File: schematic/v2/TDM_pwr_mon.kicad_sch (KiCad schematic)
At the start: 42 parts, among them J10 INA219_CONFIG, J11 INA219_CONFIG, J15 INA219_CONFIG, J5 INA219_CONFIG, J6 INA219_CONFIG, J7 INA219_CONFIG, U10 INA219AxD, U11 INA219AxD, U12 INA219AxD, U13 INA219AxD, U20 INA219AxD, U7 INA219AxD

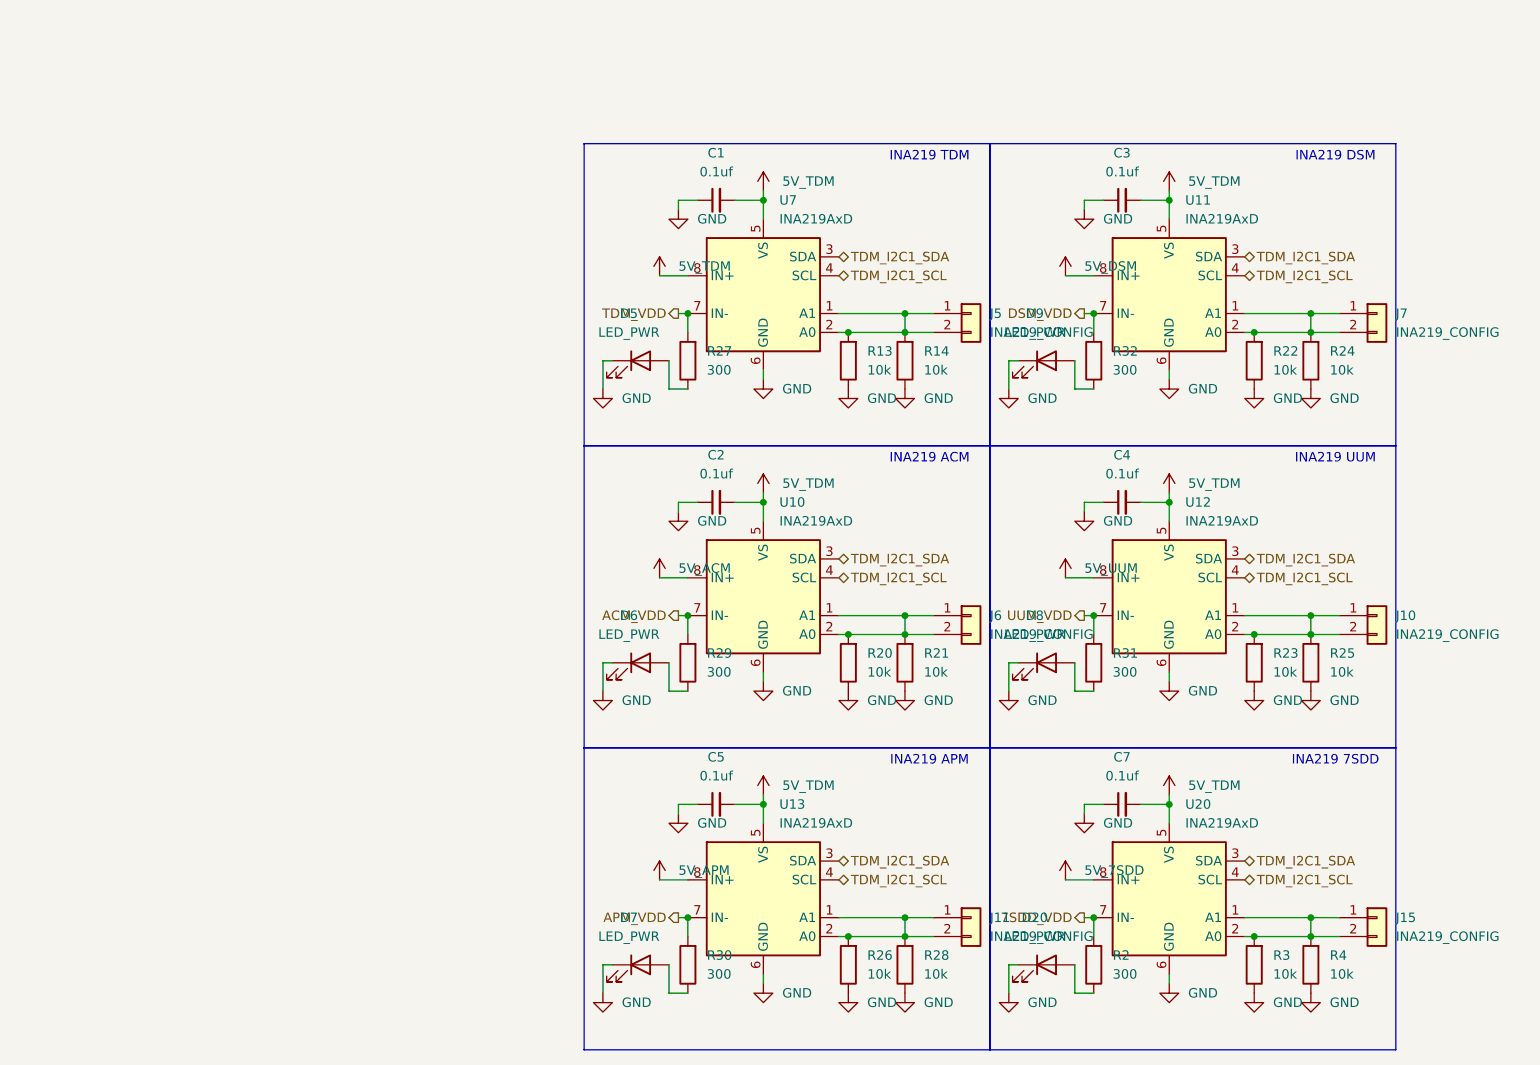
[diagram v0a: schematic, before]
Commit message: no errors in the ERC!
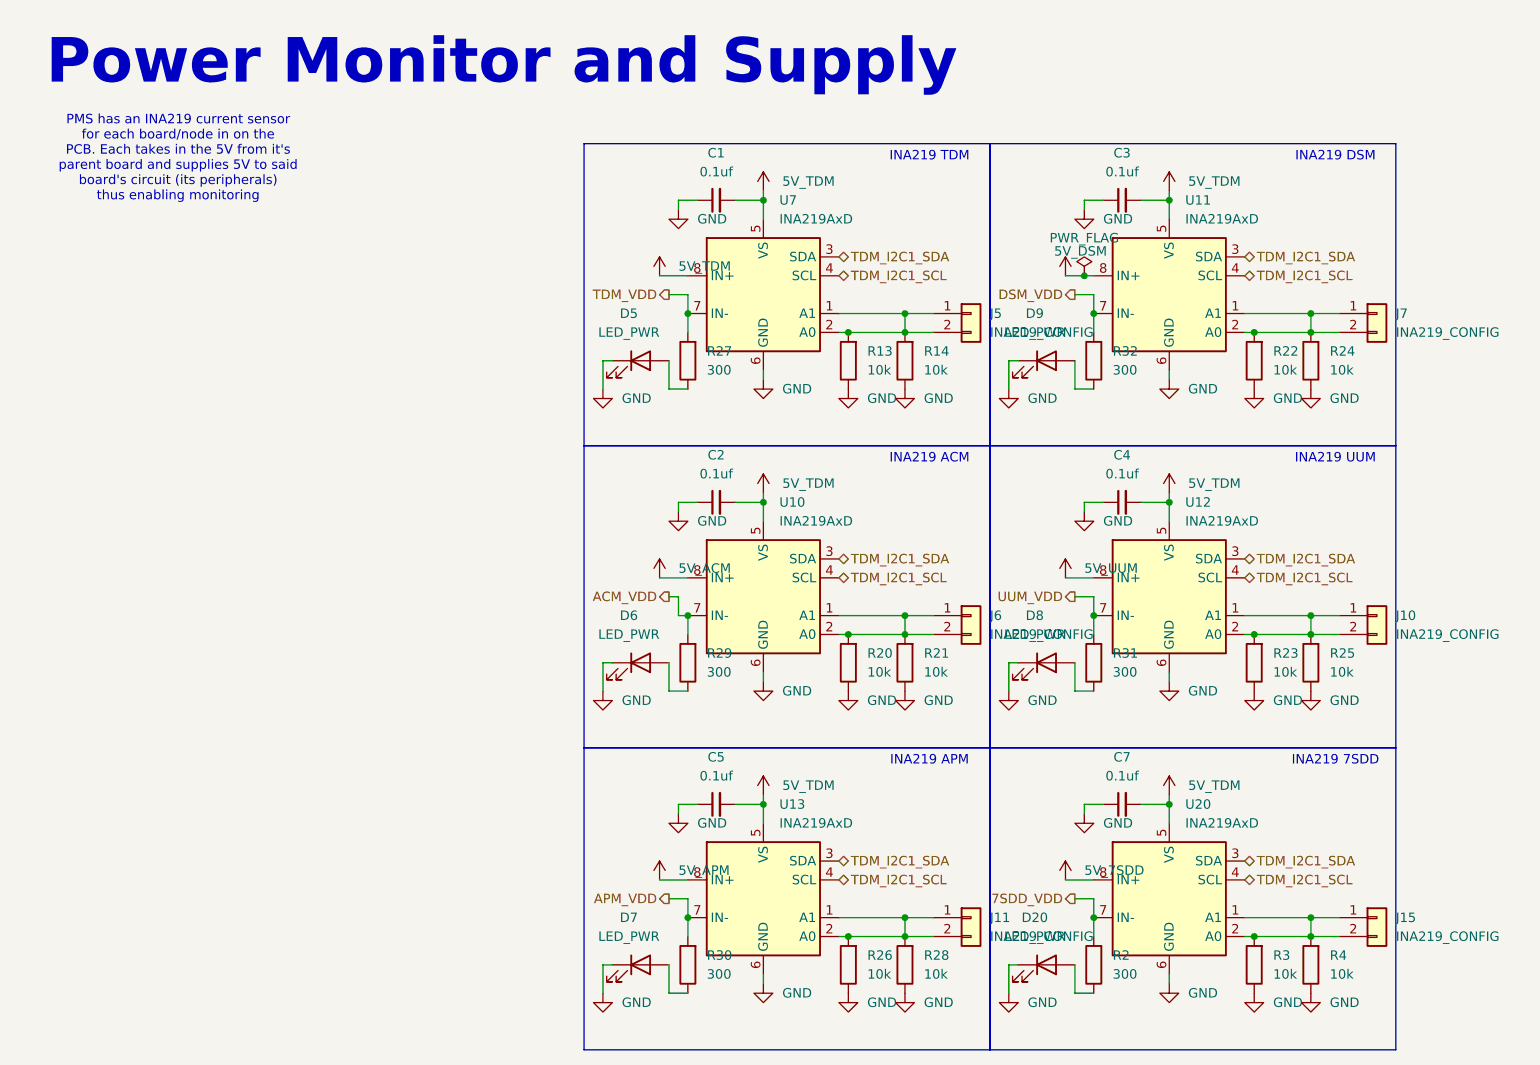
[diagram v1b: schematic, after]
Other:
- note added: "PMS has an INA219 current sensor for each board/node in on the PCB. Each takes in the 5V from it's parent board and supplies 5V to said board's circuit (its peripherals) thus enabling monitoring"
- note added: "Power Monitor and Supply"
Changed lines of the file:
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@@
 		)
 	)
+	(text "PMS has an INA219 current sensor\nfor each board/node in on the \nPCB. Each takes in the 5V from it's\nparent board and supplies 5V to said\nboard's circuit (its peripherals)\nthus enabling monitoring"
+		(exclude_from_sim no)
+		(at 34.29 32.512 0)
+		(effects
+			(font
+				(size 1.27 1.27)
+			)
+		)
+	)
 	(text "INA219 ACM"
 		(exclude_from_sim no)
@@
 		)
 	)
+	(text "Power Monitor and Supply"
+		(exclude_from_sim no)
+		(at 16.51 23.114 0)
+		(effects
+			(font
+				(size 5.9944 5.9944)
+				(thickness 1.1989)
+				(bold yes)
+			)
+			(justify left bottom)
+		)
+	)
 	(text "INA219 UUM"
 		(exclude_from_sim no)
@@
 	)
 	(junction
+		(at 156.21 48.26)
+		(diameter 0)
+		(color 0 0 0 0)
+	)
+	(junction
 		(at 186.69 93.98)
 		(diameter 0)
@@
 	(wire
 		(pts
-			(xy 153.67 48.26) (xy 157.48 48.26)
+			(xy 167.64 38.1) (xy 167.64 40.64)
+		)
+		(stroke
+			(width 0)
+			(type default)
+		)
+	)
+	(wire
+		(pts
+			(xy 153.67 48.26) (xy 156.21 48.26)
 		)
 		(stroke
@@
 	(wire
 		(pts
-			(xy 163.83 78.74) (xy 167.64 78.74)
+			(xy 156.21 48.26) (xy 157.48 48.26)
 		)
 		(stroke
@@
 	(wire
 		(pts
-			(xy 101.6 134.62) (xy 102.87 134.62)
+			(xy 157.48 132.08) (xy 157.48 134.62)
+		)
+		(stroke
+			(width 0)
+			(type default)
+		)
+	)
+	(wire
+		(pts
+			(xy 163.83 78.74) (xy 167.64 78.74)
 		)
 		(stroke
@@
 	(wire
 		(pts
+			(xy 102.87 132.08) (xy 102.87 134.62)
+		)
+		(stroke
+			(width 0)
+			(type default)
+		)
+	)
+	(wire
+		(pts
 			(xy 154.94 59.69) (xy 154.94 63.5)
 		)
@@
 	(wire
 		(pts
+			(xy 157.48 91.44) (xy 157.48 93.98)
+		)
+		(stroke
+			(width 0)
+			(type default)
+		)
+	)
+	(wire
+		(pts
 			(xy 100.33 63.5) (xy 102.87 63.5)
 		)
@@
 	(wire
 		(pts
-			(xy 156.21 53.34) (xy 157.48 53.34)
+			(xy 154.94 50.8) (xy 157.48 50.8)
 		)
 		(stroke
@@
 	(wire
 		(pts
-			(xy 167.64 118.11) (xy 167.64 119.38)
+			(xy 99.06 88.9) (xy 102.87 88.9)
 		)
 		(stroke
@@
 	(wire
 		(pts
-			(xy 177.8 137.16) (xy 179.07 137.16)
+			(xy 167.64 118.11) (xy 167.64 119.38)
 		)
 		(stroke
@@
 	(wire
 		(pts
-			(xy 113.03 101.6) (xy 113.03 102.87)
+			(xy 177.8 137.16) (xy 179.07 137.16)
 		)
 		(stroke
@@
 	(wire
 		(pts
-			(xy 123.19 96.52) (xy 124.46 96.52)
+			(xy 113.03 101.6) (xy 113.03 102.87)
 		)
 		(stroke
@@
 	(wire
 		(pts
-			(xy 153.67 88.9) (xy 157.48 88.9)
+			(xy 123.19 96.52) (xy 124.46 96.52)
 		)
 		(stroke
@@
 	(wire
 		(pts
-			(xy 167.64 38.1) (xy 167.64 40.64)
-		)
-		(stroke
-			(width 0)
-			(type default)
-		)
-	)
-	(wire
-		(pts
 			(xy 91.44 100.33) (xy 92.71 100.33)
 		)
@@
 	(wire
 		(pts
-			(xy 156.21 134.62) (xy 157.48 134.62)
+			(xy 154.94 132.08) (xy 157.48 132.08)
 		)
 		(stroke
@@
 	(wire
 		(pts
-			(xy 156.21 93.98) (xy 157.48 93.98)
+			(xy 154.94 91.44) (xy 157.48 91.44)
 		)
 		(stroke
@@
 	(wire
 		(pts
-			(xy 101.6 53.34) (xy 102.87 53.34)
+			(xy 100.33 50.8) (xy 102.87 50.8)
 		)
 		(stroke
@@
 	(wire
 		(pts
-			(xy 101.6 93.98) (xy 102.87 93.98)
+			(xy 100.33 91.44) (xy 101.6 91.44)
 		)
 		(stroke
@@
 	(wire
 		(pts
+			(xy 102.87 132.08) (xy 100.33 132.08)
+		)
+		(stroke
+			(width 0)
+			(type default)
+		)
+	)
+	(wire
+		(pts
 			(xy 186.69 53.34) (xy 190.5 53.34)
 		)
@@
 	(wire
 		(pts
+			(xy 102.87 50.8) (xy 102.87 53.34)
+		)
+		(stroke
+			(width 0)
+			(type default)
+		)
+	)
+	(wire
+		(pts
 			(xy 156.21 38.1) (xy 158.75 38.1)
 		)
@@
 	(wire
 		(pts
+			(xy 101.6 91.44) (xy 101.6 93.98)
+		)
+		(stroke
+			(width 0)
+			(type default)
+		)
+	)
+	(wire
+		(pts
 			(xy 91.44 140.97) (xy 92.71 140.97)
 		)
@@
 	(wire
 		(pts
+			(xy 101.6 93.98) (xy 102.87 93.98)
+		)
+		(stroke
+			(width 0)
+			(type default)
+		)
+	)
+	(wire
+		(pts
 			(xy 179.07 137.16) (xy 186.69 137.16)
 		)
@@
 	(wire
 		(pts
+			(xy 153.67 88.9) (xy 157.48 88.9)
+		)
+		(stroke
+			(width 0)
+			(type default)
+		)
+	)
+	(wire
+		(pts
 			(xy 91.44 59.69) (xy 92.71 59.69)
 		)
@@
 	(wire
 		(pts
-			(xy 99.06 88.9) (xy 102.87 88.9)
-		)
-		(stroke
-			(width 0)
-			(type default)
-		)
-	)
-	(wire
-		(pts
 			(xy 132.08 53.34) (xy 135.89 53.34)
 		)
@@
 	(wire
 		(pts
+			(xy 157.48 50.8) (xy 157.48 53.34)
+		)
+		(stroke
+			(width 0)
+			(type default)
+		)
+	)
+	(wire
+		(pts
 			(xy 157.48 137.16) (xy 157.48 134.62)
 		)
@@
 	(hierarchical_label "DSM_VDD"
 		(shape output)
-		(at 156.21 53.34 180)
+		(at 154.94 50.8 180)
 		(effects
 			(font
@@
 	(hierarchical_label "UUM_VDD"
 		(shape output)
-		(at 156.21 93.98 180)
+		(at 154.94 91.44 180)
 		(effects
 			(font
@@
 	(hierarchical_label "TDM_VDD"
 		(shape output)
-		(at 101.6 53.34 180)
+		(at 100.33 50.8 180)
 		(effects
 			(font
@@
 	(hierarchical_label "7SDD_VDD"
 		(shape output)
-		(at 156.21 134.62 180)
+		(at 154.94 132.08 180)
 		(effects
 			(font
@@
 	(hierarchical_label "APM_VDD"
 		(shape output)
-		(at 101.6 134.62 180)
+		(at 100.33 132.08 180)
 		(effects
 			(font
@@
 	(hierarchical_label "ACM_VDD"
 		(shape output)
-		(at 101.6 93.98 180)
+		(at 100.33 91.44 180)
 		(effects
 			(font
@@
 	)
 	(symbol
+		(lib_id "power:PWR_FLAG")
+		(at 156.21 48.26 0)
+		(unit 1)
+		(exclude_from_sim no)
+		(in_bom yes)
+		(on_board yes)
+		(dnp no)
+		(fields_autoplaced yes)
+		(property "Reference" "#FLG012"
+			(at 156.21 46.355 0)
+			(effects
+				(font
+					(size 1.27 1.27)
+				)
+				(hide yes)
+			)
+		)
+		(property "Value" "PWR_FLAG"
+			(at 156.21 43.18 0)
+			(effects
+				(font
+					(size 1.27 1.27)
+				)
+			)
+		)
+		(property "Footprint" ""
+			(at 156.21 48.26 0)
+			(effects
+				(font
+					(size 1.27 1.27)
+				)
+				(hide yes)
+			)
+		)
+		(property "Datasheet" "~"
+			(at 156.21 48.26 0)
+			(effects
+				(font
+					(size 1.27 1.27)
+				)
+				(hide yes)
+			)
+		)
+		(property "Description" "Special symbol for telling ERC where power comes from"
+			(at 156.21 48.26 0)
+			(effects
+				(font
+					(size 1.27 1.27)
+				)
+				(hide yes)
+			)
+		)
+		(pin "1"
+		)
+		(instances
+			(project ""
+				(path "/fe7b15e9-f0ed-4338-9f03-dd7651dace13/442c7b41-f8c0-48e5-8b80-63d502cac366/c9161959-85ce-4cf5-b3d5-3776fec616f5"
+					(reference "#FLG012")
+					(unit 1)
+				)
+			)
+		)
+	)
+	(symbol
 		(lib_id "power:+5V")
 		(at 113.03 77.47 0)
@@
 		(on_board yes)
 		(dnp no)
-		(fields_autoplaced yes)
 		(property "Reference" "#PWR050"
 			(at 153.67 52.07 0)
@@
 		)
 		(property "Value" "5V_DSM"
-			(at 156.21 46.9899 0)
+			(at 152.146 44.958 0)
 			(effects
 				(font
